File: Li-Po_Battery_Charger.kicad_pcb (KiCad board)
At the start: 2 copper layers, 46 x 24.2 mm, 39 parts, among them Q1 FS8205A_C908265, U1 DW01A, U2 MP1584EN-LF-Z, U3 MCP73871-2CCI/ML

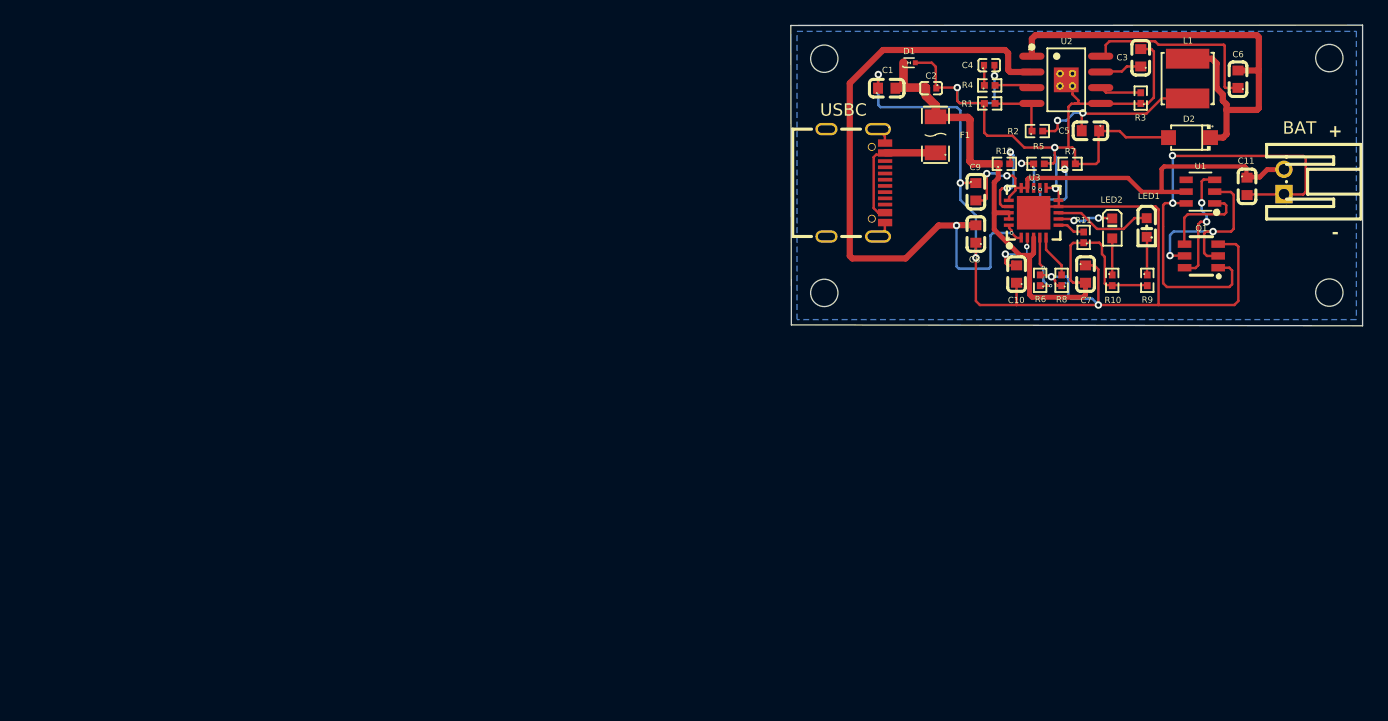
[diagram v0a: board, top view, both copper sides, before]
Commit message: Final Production Version
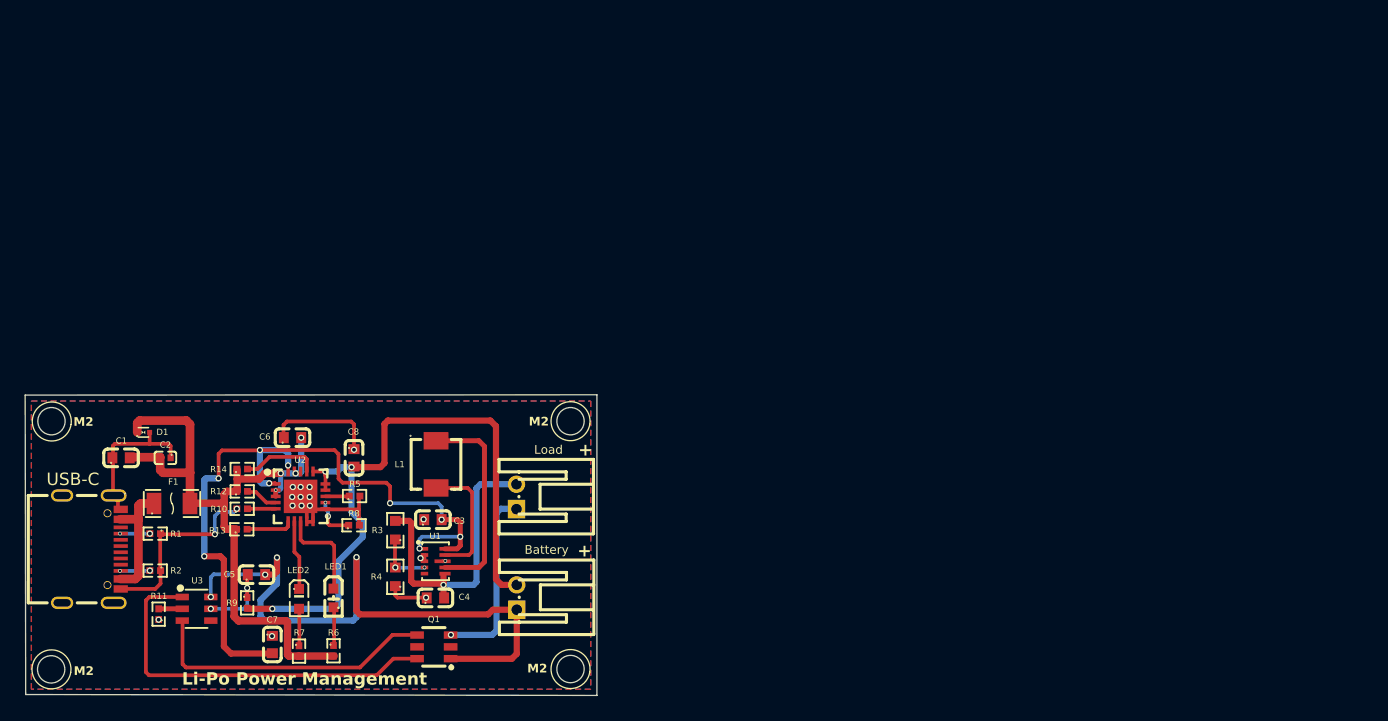
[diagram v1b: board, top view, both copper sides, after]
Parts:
- removed BAT: S2B-PH-K-S(LF)(SN), lcsc_footprints:C173752_CONN-TH_S2B-PH-K-S-LF-SN
- removed C10: 10uF, lcsc_footprints:C22392391_C0603
- removed C11: 100nF, lcsc_footprints:C5137616_C0603
- removed C9: 10uF, lcsc_footprints:C3039641_C0603
- removed D2: SS34L, lcsc_footprints:C3003093_SMF_L2_8-W1_8-LS3_7-RD
- removed REF** (x4): MountingHole_2.2mm_M2_DIN965, MountingHole:MountingHole_2.2mm_M2_DIN965
- removed USBC: TYPE-C 16P(073), lcsc_footprints:C668624_USB-C-SMD_TYPE-C16PIN_C668624
- added ?: , , F.Cu at (155.0, 83.0)
- added ?: , , F.Cu at (113.2, 83.0)
- added ?: , , F.Cu at (113.2, 103.0)
- added ?: , , F.Cu at (155.0, 103.0)
- added Battery: S2B-PH-K-S(LF)(SN), lcsc_footprints:C173752_CONN-TH_S2B-PH-K-S-LF-SN, F.Cu at (150.7, 97.2)
- added Load: S2B-PH-K-S(LF)(SN), lcsc_footprints:C173752_CONN-TH_S2B-PH-K-S-LF-SN, F.Cu at (150.7, 89.1)
- added R13: 10kΩ, lcsc_footprints:C326912_R0402, F.Cu at (128.5, 91.8)
- added R14: 10kΩ, lcsc_footprints:C326912_R0402, F.Cu at (128.6, 86.9)
- added USB-C: TYPE-C 16P(073), lcsc_footprints:C668624_USB-C-SMD_TYPE-C16PIN_C668624, F.Cu at (116.4, 93.3)
- C3: value 22uF -> 10uF; footprint lcsc_footprints:C22367828_C0603 -> lcsc_footprints:C3039641_C0603
- C4: value 10nF -> 22uF; footprint lcsc_footprints:C15195_C0402 -> lcsc_footprints:C22367828_C0603
- C5: value 22uF -> 100nF; footprint lcsc_footprints:C22367828_C0603 -> lcsc_footprints:C5137616_C0603
- C6: value 100nF -> 10uF; footprint lcsc_footprints:C5137616_C0603 -> lcsc_footprints:C3039641_C0603
- F1: value 0.50A 24V -> 1.5A; footprint lcsc_footprints:C70076_F1206 -> lcsc_footprints:C118413_F1206
- L1: value YNR4030-4R7M -> 0.47 µH; footprint lcsc_footprints:C340391_IND-SMD_L4_0-W4_0 -> lcsc_footprints:C285747_IND-SMD_L4_0-W4_0_CHILISIN_MHCI04012N
- R1: value 10kΩ -> 5.1KΩ; footprint lcsc_footprints:C326912_R0402 -> lcsc_footprints:C25905_R0402
- R10: value 1KΩ -> 10kΩ; footprint lcsc_footprints:C11702_R0402 -> lcsc_footprints:C326912_R0402
- R11: value 10kΩ -> 1KΩ; footprint lcsc_footprints:C326912_R0402 -> lcsc_footprints:C11702_R0402
- R2: value RMC040231.6K1%N -> 5.1KΩ; footprint lcsc_footprints:C325374_R0402 -> lcsc_footprints:C25905_R0402
- R3: value 100KΩ -> 511kΩ; footprint lcsc_footprints:C60491_R0402 -> lcsc_footprints:C861454_R0603
- R4: value 10kΩ -> 91 kΩ; footprint lcsc_footprints:C326912_R0402 -> lcsc_footprints:C2907077_R0603
- R7: value 100KΩ -> 1KΩ; footprint lcsc_footprints:C60491_R0402 -> lcsc_footprints:C11702_R0402
- R8: value 10kΩ -> 20 kΩ; footprint lcsc_footprints:C326912_R0402 -> lcsc_footprints:C93942_R0402
- R9: value 1KΩ -> 100Ω; footprint lcsc_footprints:C11702_R0402 -> lcsc_footprints:C106232_R0402
- U1: value DW01A -> TPS63802DLAR; footprint lcsc_footprints:C42459937_SOT-23-6_L2_9-W1_6-P0_95-LS2_8-BL -> lcsc_footprints:C2845237_VSON-10_L3_0-W2_0-P0_50-TL
- U2: value MP1584EN-LF-Z -> MCP73871-2CCI/ML; footprint lcsc_footprints:C15051_SOIC-8_L5_0-W4_0-P1_27-LS6_0-BL-EP2_0 -> lcsc_footprints:C5121473_QFN-20_L4_0-W4_0-P0_50-BL-EP2_7
- U3: value MCP73871-2CCI/ML -> DW01A; footprint lcsc_footprints:C5121473_QFN-20_L4_0-W4_0-P0_50-BL-EP2_7 -> lcsc_footprints:C42459937_SOT-23-6_L2_9-W1_6-P0_95-LS2_8-BL
- moved C6 81.4 mm to (132.6, 84.4), turned to 0 degrees
- moved R11 80.4 mm to (121.8, 98.6)
- moved R2 79.3 mm to (121.6, 95.1), turned to 180 degrees
- moved R9 77.0 mm to (129.0, 97.7)
- moved C5 76.0 mm to (129.7, 95.4), turned to 0 degrees
- moved R1 75.6 mm to (121.6, 92.1), turned to 180 degrees
- moved U3 74.5 mm to (124.9, 98.2), turned to -90 degrees
- moved R7 73.4 mm to (133.2, 101.6), turned to -90 degrees
- moved R10 72.4 mm to (128.6, 90.1), turned to 0 degrees
- moved C7 71.9 mm to (131.0, 101.0)
- moved LED1 71.9 mm to (135.9, 97.3)
- moved LED2 71.9 mm to (133.2, 97.3)
- moved U2 70.2 mm to (133.3, 89.1)
- moved R3 69.3 mm to (140.9, 91.8)
- moved Q1 69.3 mm to (144.0, 101.2)
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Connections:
- C3 pad 1: Net-(U2-VIN) -> GND
- C3 pad 2: GND -> /VSYS
- C4 pad 1: Net-(C4-Pad1) -> GND
- C4 pad 2: GND -> /3.3V
- C5 pad 1: GND -> Net-(U3-VDD)
- C5 pad 2: /3.3V -> /B-
- C6 pad 1: Net-(U2-BST) -> GND
- C6 pad 2: Net-(D2-C) -> /+5V_USB
- C7 pad 2: /+5V_USB -> /VSYS
- C8 pad 2: /VSYS -> /VBAT
- L1 pad 1: /3.3V -> Net-(U1-L2)
- L1 pad 2: Net-(D2-C) -> Net-(U1-L1)
- Q1 pad 2: /CSI -> unconnected-(Q1-D1/D2-Pad2)
- Q1 pad 4: /OD -> /OC
- Q1 pad 5: /CSI -> unconnected-(Q1-D1/D2-Pad5)
- Q1 pad 6: /OC -> /OD
- R1 pad 2: Net-(U2-FB) -> /CC1
- R10 pad 1: Net-(LED2-A) -> GND
- R10 pad 2: /+5V_USB -> /THERM
- R11 pad 1: /+5V_USB -> GND
- R11 pad 2: /PG# -> /CSI
- R12 pad 2: /CE -> /PROG2
- R2 pad 1: Net-(U2-FB) -> GND
- R2 pad 2: /3.3V -> /CC2
- R3 pad 1: GND -> Net-(U1-FB)
- R3 pad 2: Net-(U2-FREQ) -> /3.3V
- R4 pad 1: Net-(C4-Pad1) -> GND
- R4 pad 2: Net-(U2-COMP) -> Net-(U1-FB)
- R6 pad 1: /PROG2 -> Net-(LED1-A)
- R6 pad 2: GND -> /+5V_USB
- R7 pad 1: /PROG3 -> Net-(LED2-A)
- R7 pad 2: GND -> /+5V_USB
- R8 pad 1: GND -> /PROG3
- R8 pad 2: /THERM -> GND
- R9 pad 1: Net-(LED1-A) -> Net-(U3-VDD)
- R9 pad 2: /+5V_USB -> /VBAT
- U1 pad 1: /OD -> /VSYS
- U1 pad 2: /CSI -> GND
- U1 pad 3: /OC -> GND
- U1 pad 4: unconnected-(U1-NC-Pad4) -> Net-(U1-FB)
- U1 pad 5: /VBAT -> unconnected-(U1-PG-Pad5)
- U1 pad 6: /B- -> /3.3V
- U2 pad 1: Net-(D2-C) -> /VSYS
- U2 pad 2: /VSYS -> /+5V_USB
- U2 pad 3: Net-(U2-COMP) -> /+5V_USB
- U2 pad 4: Net-(U2-FB) -> /PROG2
- U2 pad 5: GND -> /THERM
- U2 pad 6: Net-(U2-FREQ) -> /PG#
- U2 pad 7: Net-(U2-VIN) -> /STAT2
- U2 pad 8: Net-(U2-BST) -> /STAT1
- U3 pad 1: /VSYS -> /OD
- U3 pad 2: /VPCC -> /CSI
- U3 pad 3: /+5V_USB -> /OC
- U3 pad 4: /PROG2 -> unconnected-(U3-NC-Pad4)
- U3 pad 5: /THERM -> Net-(U3-VDD)
- U3 pad 6: /PG# -> /B-
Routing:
- net GND: track 154.0 -> 66.4 mm, vias 9 -> 19
- net Net-(D2-C): track 39.8 -> 0.00 mm
- net /OD: track 7.26 -> 31.3 mm
- net /VBAT: track 35.3 -> 54.4 mm, vias 2 -> 3
- net Net-(U1-L2): track 0.00 -> 16.8 mm
- net Net-(U2-BST): track 15.2 -> 0.00 mm
- net /CSI: track 16.2 -> 1.90 mm, vias 2 -> 0
- net /B-: track 38.7 -> 52.8 mm, vias 2 -> 4
- net /OC: track 9.79 -> 23.6 mm, vias 2 -> 0
- net Net-(U1-L1): track 0.00 -> 10.1 mm
- net /3.3V: track 14.6 -> 24.3 mm, vias 2 -> 1
- net /VSYS: track 54.7 -> 61.8 mm, vias 2 -> 9
- net Net-(U3-VDD): track 0.00 -> 6.33 mm, vias 0 -> 2
- net Net-(U2-FB): track 5.22 -> 0.00 mm
- net /VPCC: track 5.15 -> 0.00 mm, vias 2 -> 0
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- added copper zone on F.Cu, net GND
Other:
- board text added: "Li-Po Power Management"
- board text added: "M2"
- board text removed: "-"
